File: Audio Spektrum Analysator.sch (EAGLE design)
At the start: 148 parts, among them IC1 LM324N, IC10 LM3914N, IC11 LM3914N, IC12 LM3914N, IC13 LM3914N, IC2 LM324N, IC3 LM324N, IC4 LM3914N, IC5 LM3914N, IC6 LM3914N, IC7 LM3914N, IC8 LM3914N, IC9 LM3914N, J2 DCJ0202, M1 ELECTRET_MICROPHON-F6050AP

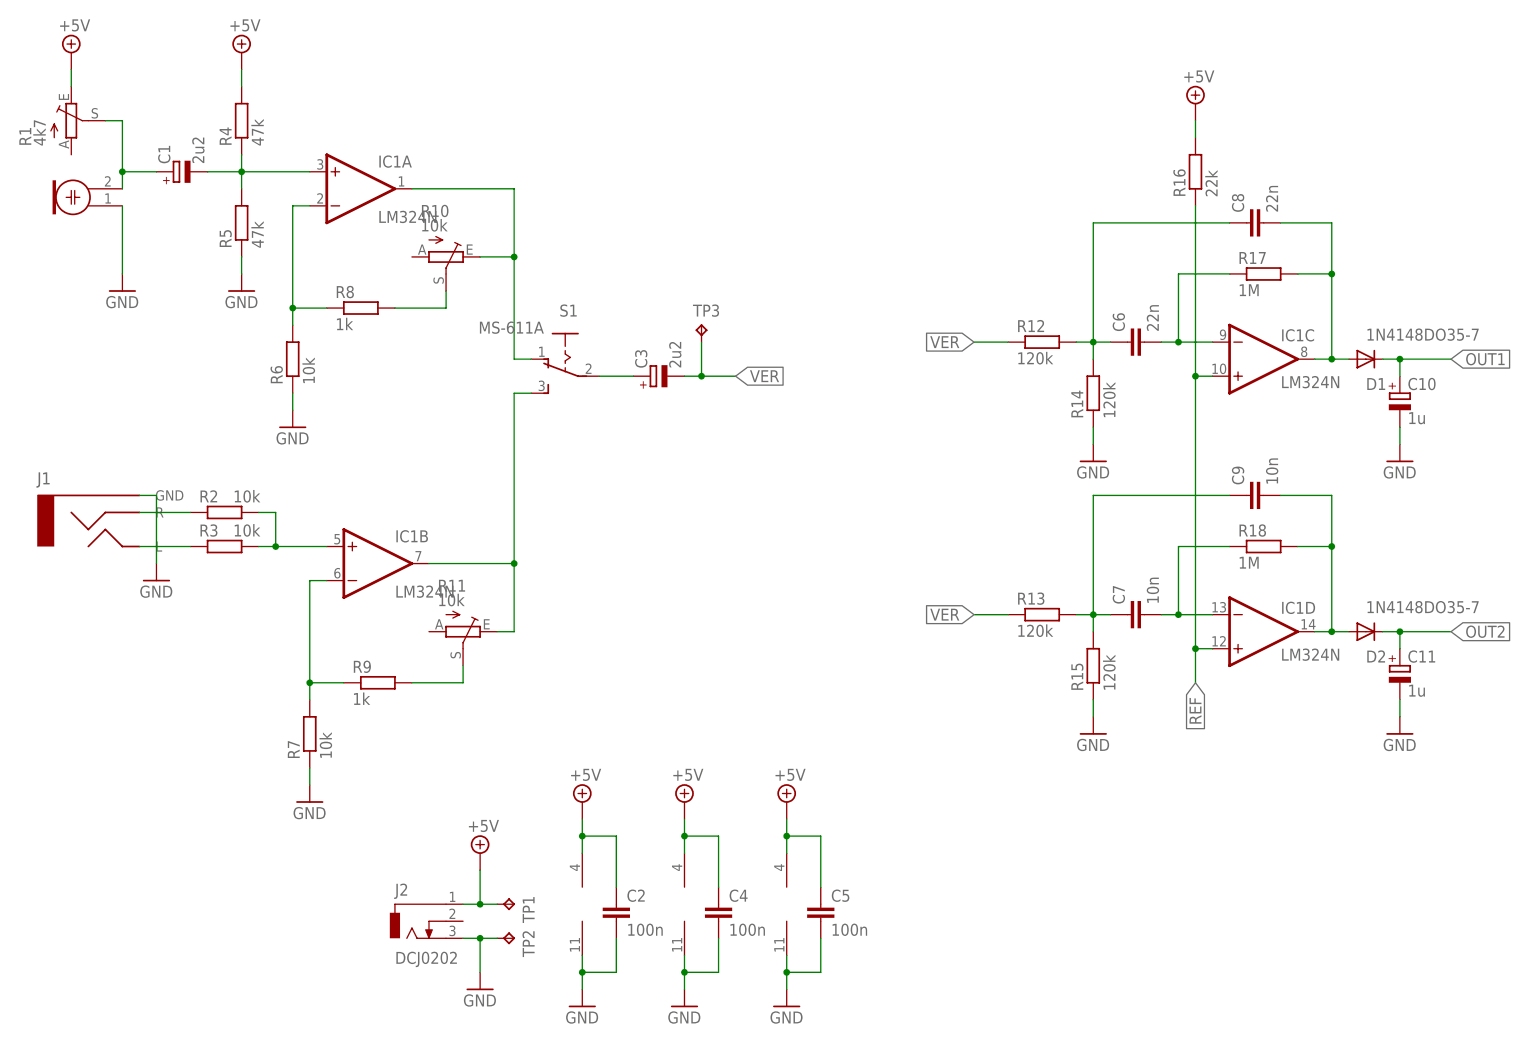
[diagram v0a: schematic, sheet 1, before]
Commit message: moved names
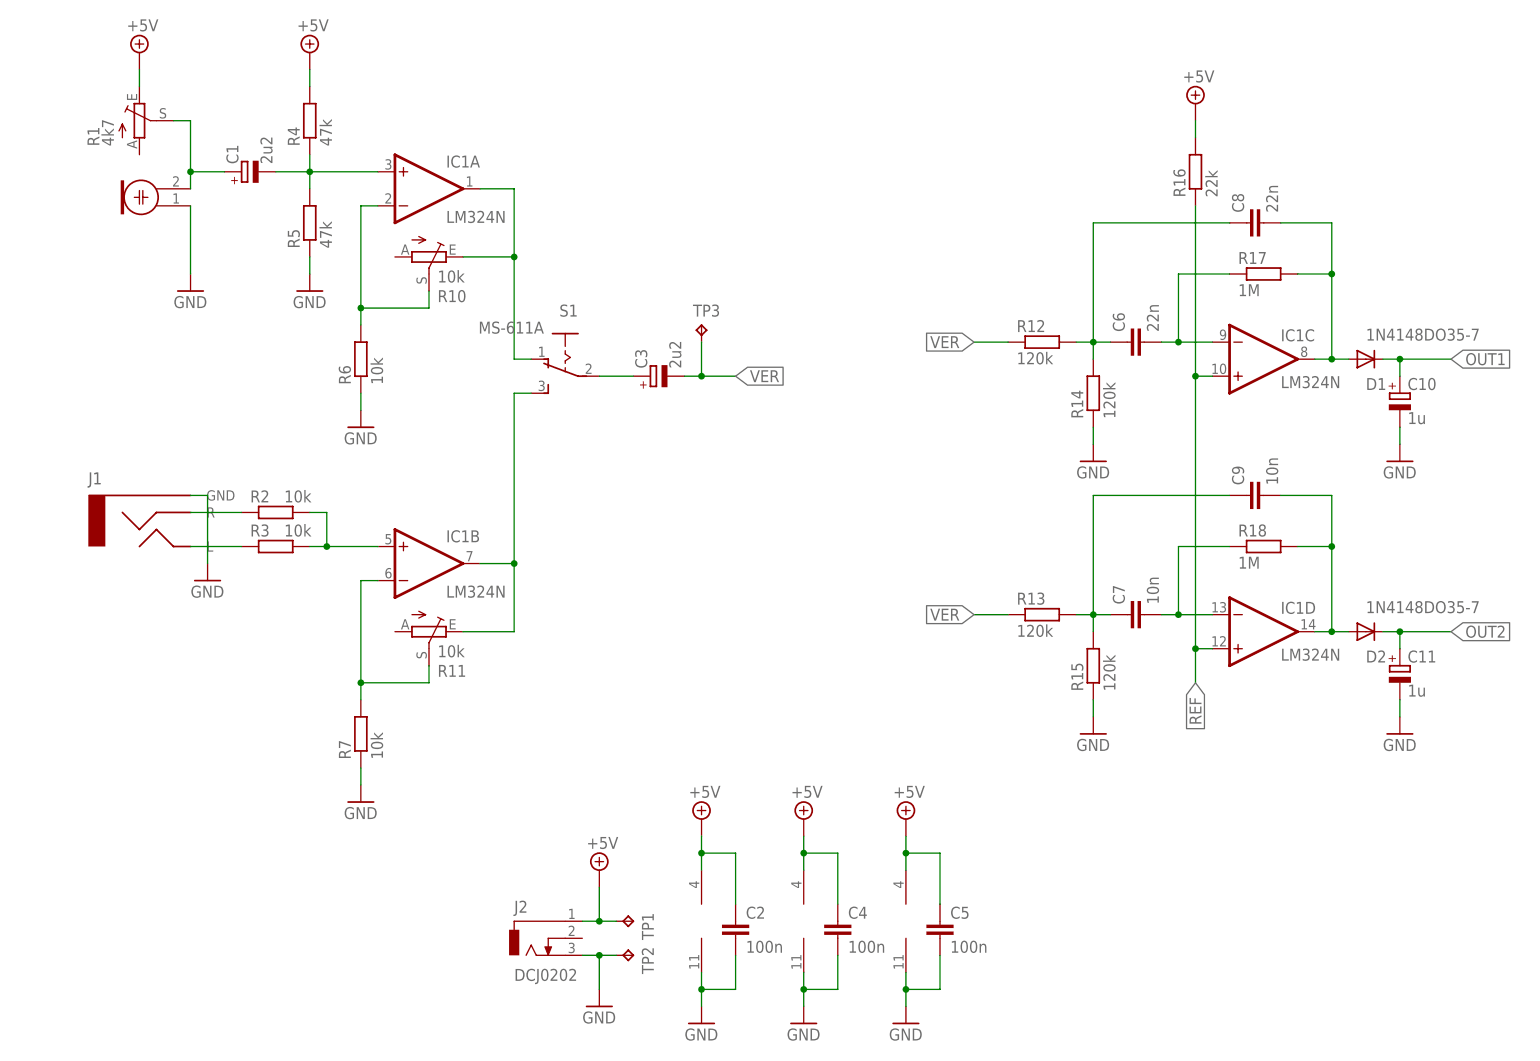
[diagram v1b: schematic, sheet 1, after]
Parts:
- removed R8: 1k, rcl:R-EU_0207/7
- removed R9: 1k, resistor:R-EU_0207/7
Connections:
- removed net N$31: R10.S, R8.2
- removed net N$44: R11.S, R9.2
- net N$123: now also R11.S; no longer R9.1
- net N$5: now also R10.S; no longer R8.1
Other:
- moved on the sheet: C1, C2, C4, C5, IC1A, IC1B, J1, J2, R1, R10, R11, R2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
